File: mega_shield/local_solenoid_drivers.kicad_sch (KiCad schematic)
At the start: 10 parts, among them J7 1803277, Q43 AO4486, U29 NUP2202

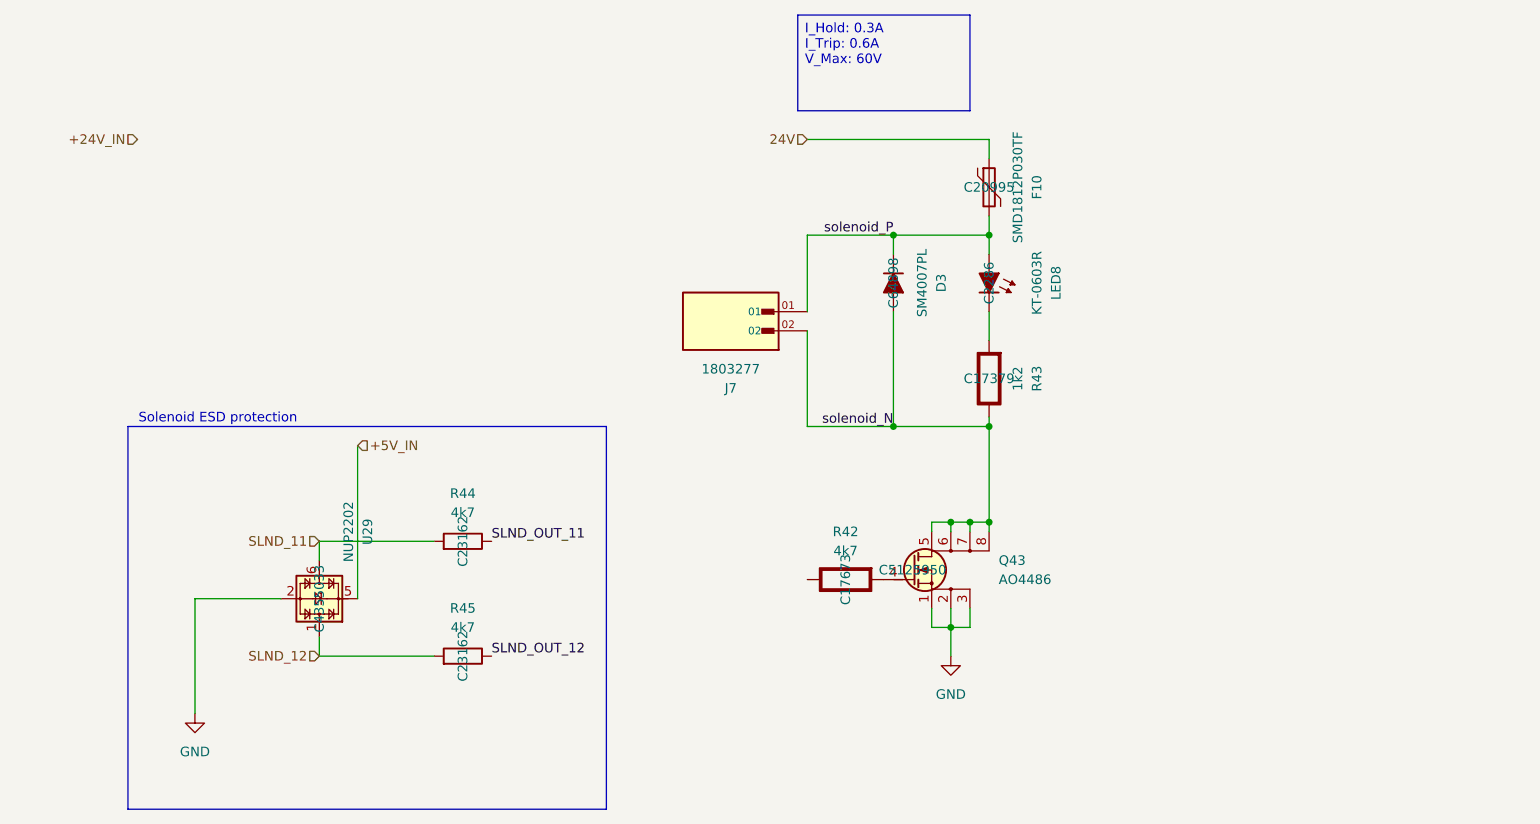
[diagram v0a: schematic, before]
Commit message: finished adding the local solenoid dirver's
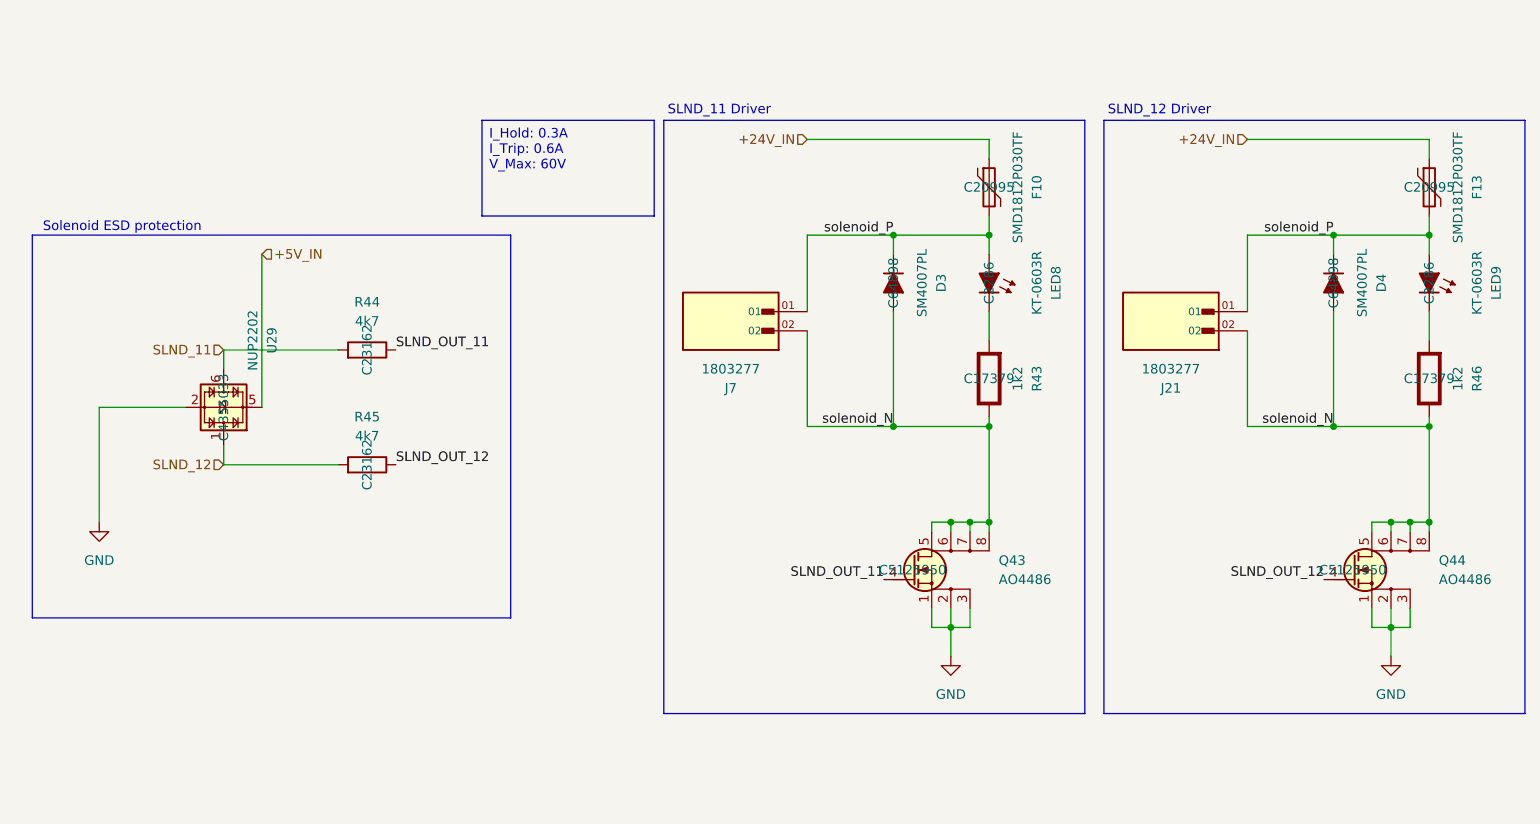
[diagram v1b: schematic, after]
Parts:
- removed R42: 4k7, Resistor_SMD:R_0805_2012Metric_Pad1.20x1.40mm_HandSolder, symbol PCM_Elektuur:R
- added D4: SM4007PL, PCM_Diode_SMD_AKL:D_SOD-123F, symbol PCM_Diode_AKL:SM4007PL
- added F13: SMD1812P030TF, Fuse:Fuse_1812_4532Metric_Pad1.30x3.40mm_HandSolder, symbol Device:Polyfuse
- added J21: 1803277, footprints:PHOENIX_1803277, symbol TERM_BLOCK_HDR_2POS_3.81MM:1803277
- added LED9: KT-0603R, PCM_LED_SMD_AKL:LED_0201_0603Metric, symbol PCM_LED_AKL:LED_1.8mm_SMD
- added Q44: AO4486, PCM_Package_SO_AKL:SO-8_3.9x4.9mm_P1.27mm, symbol PCM_Transistor_MOSFET_AKL:AO4486
- added R46: 1k2, Resistor_SMD:R_0805_2012Metric_Pad1.20x1.40mm_HandSolder, symbol PCM_Elektuur:R
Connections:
- net 24V is gone; now on net +24V_IN: F10.1
- net +24V_IN: now also F13.1
- net GND: now also Q44.1 (S), Q44.2 (S), Q44.3 (S)
- net SLND_OUT_11: now also Q43.4 (G)
- net SLND_OUT_12: now also Q44.4 (G)
- net solenoid_N: now also D4.2 (A), J21.02, Q44.5 (D), Q44.6 (D), Q44.7 (D), Q44.8 (D), R46.1 (+)
- net solenoid_P: now also D4.1 (K), F13.2, J21.01, LED9.2 (A)
- new net: LED9.1 (K), R46.2 (-)
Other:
- note added: "SLND_11 Driver"
- note added: "SLND_12 Driver"
- moved on the sheet: R44, R45, U29
